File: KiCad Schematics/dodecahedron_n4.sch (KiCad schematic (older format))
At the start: 65 parts, among them J1 Conn_01x04_Female, U1 IS31FL3733-QF, U2 Board, U3 Board, U4 Jumper4, U5 Jumper4

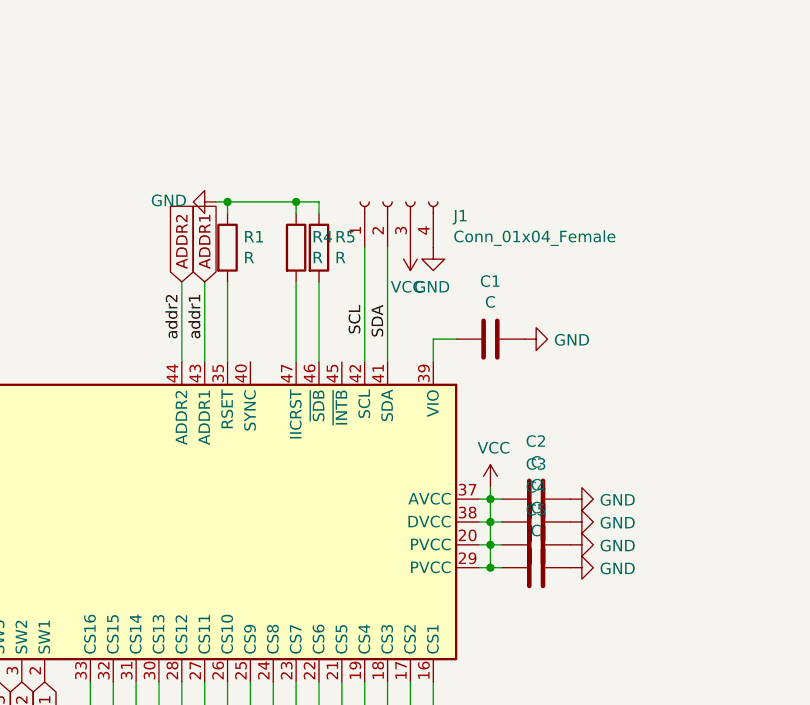
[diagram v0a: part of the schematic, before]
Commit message: moved files and final order
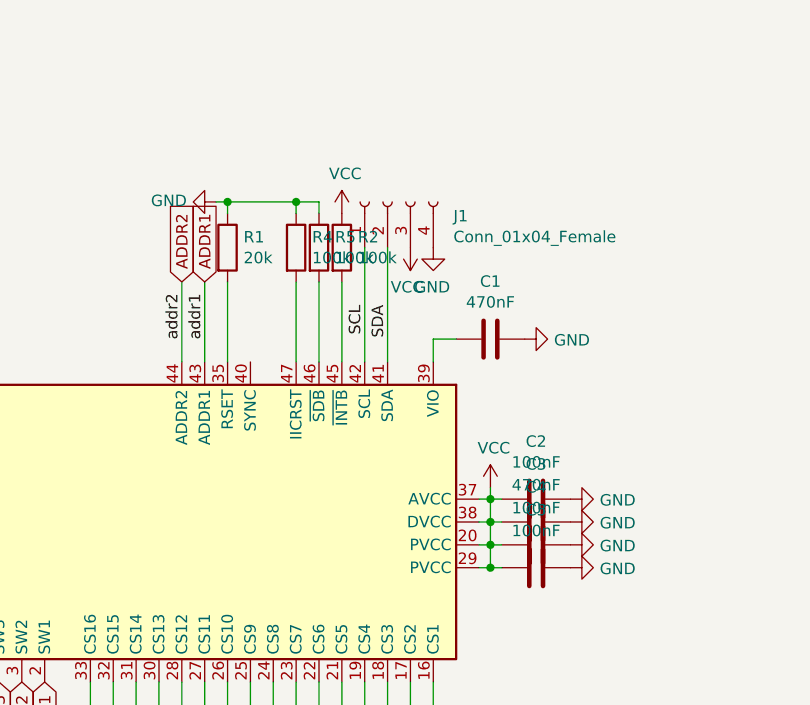
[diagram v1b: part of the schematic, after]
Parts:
- added R2: 100k, Resistor_SMD:R_0402_1005Metric_Pad0.72x0.64mm_HandSolder, symbol Device:R
- C1, C3: value C -> 470nF
- C2, C4, C5: value C -> 100nF
- R1: value R -> 20k
- R4, R5: value R -> 100k
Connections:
- net VCC: now also R2.1
- net at U1.45 (~INTB): now also R2.2
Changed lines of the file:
@@
 P 7250 -100
 F 0 "C1" V 6998 -100 50  0000 C CNN
-F 1 "C" V 7089 -100 50  0000 C CNN
+F 1 "470nF" V 7089 -100 50  0000 C CNN
 F 2 "Capacitor_SMD:C_0402_1005Metric_Pad0.74x0.62mm_HandSolder" H 7288 -250 50  0001 C CNN
 F 3 "~" H 7250 -100 50  0001 C CNN
@@
 P 6100 -500
 F 0 "R1" H 6170 -454 50  0000 L CNN
-F 1 "R" H 6170 -545 50  0000 L CNN
+F 1 "20k" H 6170 -545 50  0000 L CNN
 F 2 "Resistor_SMD:R_0402_1005Metric_Pad0.72x0.64mm_HandSolder" V 6030 -500 50  0001 C CNN
 F 3 "~" H 6100 -500 50  0001 C CNN
@@
 P 6500 -500
 F 0 "R5" H 6570 -454 50  0000 L CNN
-F 1 "R" H 6570 -545 50  0000 L CNN
+F 1 "100k" H 6570 -545 50  0000 L CNN
 F 2 "Resistor_SMD:R_0402_1005Metric_Pad0.72x0.64mm_HandSolder" V 6430 -500 50  0001 C CNN
 F 3 "~" H 6500 -500 50  0001 C CNN
@@
 P 6400 -500
 F 0 "R4" H 6470 -454 50  0000 L CNN
-F 1 "R" H 6470 -545 50  0000 L CNN
+F 1 "100k" H 6470 -545 50  0000 L CNN
 F 2 "Resistor_SMD:R_0402_1005Metric_Pad0.72x0.64mm_HandSolder" V 6330 -500 50  0001 C CNN
 F 3 "~" H 6400 -500 50  0001 C CNN
@@
 P 7450 600
 F 0 "C2" V 7198 600 50  0000 C CNN
-F 1 "C" V 7289 600 50  0000 C CNN
+F 1 "100nF" V 7289 600 50  0000 C CNN
 F 2 "Capacitor_SMD:C_0402_1005Metric_Pad0.74x0.62mm_HandSolder" H 7488 450 50  0001 C CNN
 F 3 "~" H 7450 600 50  0001 C CNN
@@
 P 7450 700
 F 0 "C3" V 7198 700 50  0000 C CNN
-F 1 "C" V 7289 700 50  0000 C CNN
+F 1 "470nF" V 7289 700 50  0000 C CNN
 F 2 "Capacitor_SMD:C_0402_1005Metric_Pad0.74x0.62mm_HandSolder" H 7488 550 50  0001 C CNN
 F 3 "~" H 7450 700 50  0001 C CNN
@@
 P 7450 800
 F 0 "C4" V 7198 800 50  0000 C CNN
-F 1 "C" V 7289 800 50  0000 C CNN
+F 1 "100nF" V 7289 800 50  0000 C CNN
 F 2 "Capacitor_SMD:C_0402_1005Metric_Pad0.74x0.62mm_HandSolder" H 7488 650 50  0001 C CNN
 F 3 "~" H 7450 800 50  0001 C CNN
@@
 P 7450 900
 F 0 "C5" V 7198 900 50  0000 C CNN
-F 1 "C" V 7289 900 50  0000 C CNN
+F 1 "100nF" V 7289 900 50  0000 C CNN
 F 2 "Capacitor_SMD:C_0402_1005Metric_Pad0.74x0.62mm_HandSolder" H 7488 750 50  0001 C CNN
 F 3 "~" H 7450 900 50  0001 C CNN
@@
 Text GLabel 8500 -2300 2    50   Input ~ 0
 ADDR2
+$Comp
+L Device:R R2
+U 1 1 61BA98A1
+P 6600 -500
+F 0 "R2" H 6670 -454 50  0000 L CNN
+F 1 "100k" H 6670 -545 50  0000 L CNN
+F 2 "Resistor_SMD:R_0402_1005Metric_Pad0.72x0.64mm_HandSolder" V 6530 -500 50  0001 C CNN
+F 3 "~" H 6600 -500 50  0001 C CNN
+	1    6600 -500
+	1    0    0    -1
+$EndComp
+Wire Wire Line
+	6600 -350 6600 0
+$Comp
+L power:VCC #PWR0115
+U 1 1 61BC27E1
+P 6600 -650
+F 0 "#PWR0115" H 6600 -800 50  0001 C CNN
+F 1 "VCC" H 6615 -477 50  0000 C CNN
+F 2 "" H 6600 -650 50  0001 C CNN
+F 3 "" H 6600 -650 50  0001 C CNN
+	1    6600 -650
+	1    0    0    -1
+$EndComp
 $EndSCHEMATC
